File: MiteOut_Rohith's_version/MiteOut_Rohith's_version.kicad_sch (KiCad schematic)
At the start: 1 part, among them U1 ESP32-S3-WROOM-1

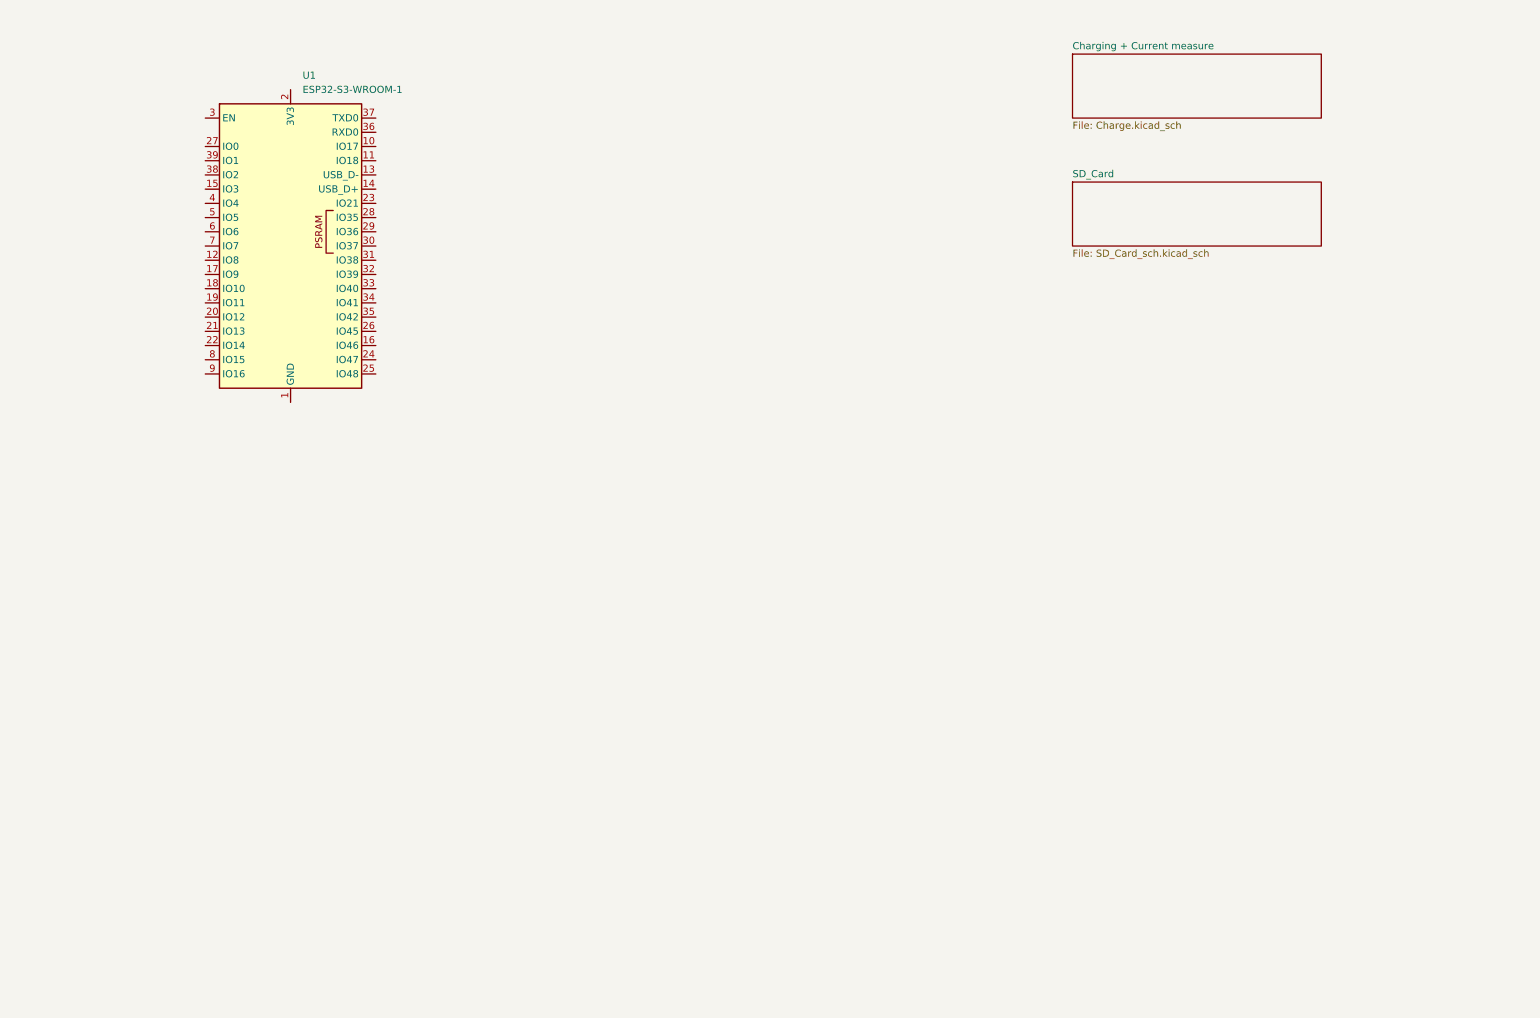
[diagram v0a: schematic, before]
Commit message: Finished ADC + ESP needing edits
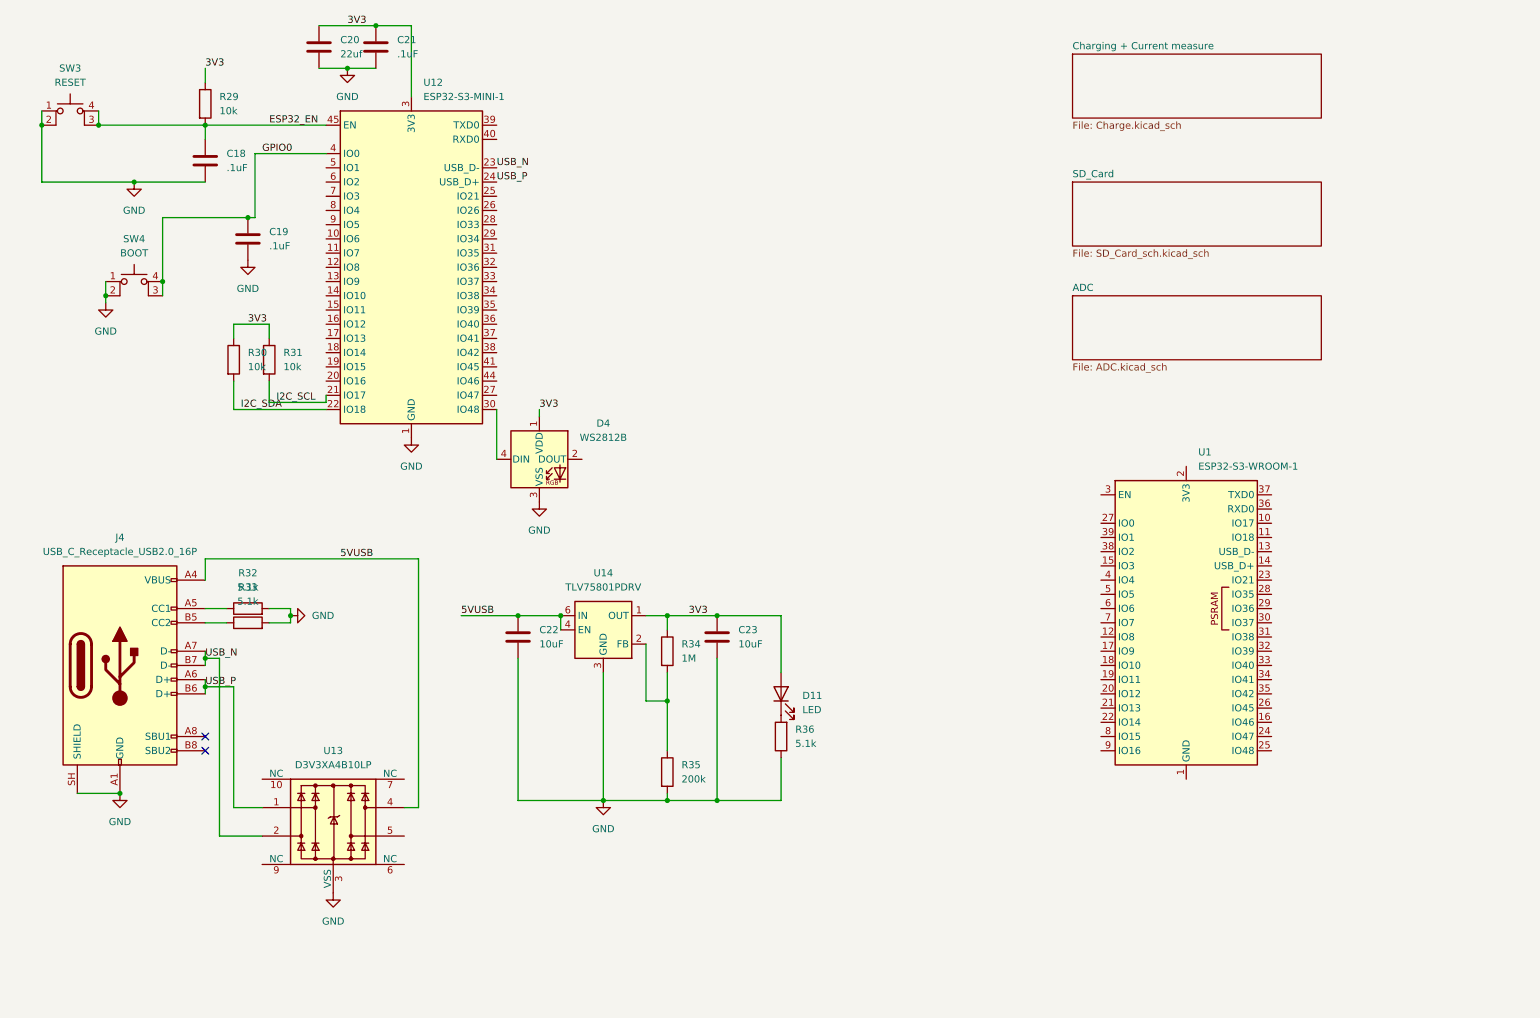
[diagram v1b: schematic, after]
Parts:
- added C18, C19, C21: .1uF, Capacitor_SMD:C_0603_1608Metric_Pad1.08x0.95mm_HandSolder, symbol Device:C
- added C20: 22uf, Capacitor_SMD:C_0603_1608Metric_Pad1.08x0.95mm_HandSolder, symbol Device:C
- added C22, C23: 10uF, symbol Device:C
- added D11: LED, LED_SMD:LED_0603_1608Metric_Pad1.05x0.95mm_HandSolder, symbol Device:LED
- added D4: WS2812B, LED_SMD:LED_WS2812B_PLCC4_5.0x5.0mm_P3.2mm, symbol LED:WS2812B
- added J4: USB_C_Receptacle_USB2.0_16P, Connector_USB:USB_C_Receptacle_GCT_USB4105-xx-A_16P_TopMnt_Horizontal, symbol Connector:USB_C_Receptacle_USB2.0_16P
- added R29, R30, R31: 10k, Resistor_SMD:R_0603_1608Metric_Pad0.98x0.95mm_HandSolder, symbol Device:R
- added R32, R33, R36: 5.1k, symbol Device:R
- added R34: 1M, Resistor_SMD:R_0603_1608Metric_Pad0.98x0.95mm_HandSolder, symbol Device:R
- added R35: 200k, Resistor_SMD:R_0603_1608Metric_Pad0.98x0.95mm_HandSolder, symbol Device:R
- added SW3: RESET, Button_Switch_SMD:SW_SPST_PTS810, symbol Switch:SW_MEC_5E
- added SW4: BOOT, Button_Switch_SMD:SW_SPST_PTS810, symbol Switch:SW_MEC_5E
- added U12: ESP32-S3-MINI-1, RF_Module:ESP32-S2-MINI-1, symbol RF_Module:ESP32-S3-MINI-1
- added U13: D3V3XA4B10LP, Package_DFN_QFN:Diodes_UDFN-10_1x2.5mm_P0.5mm, symbol Power_Protection:D3V3XA4B10LP
- added U14: TLV75801PDRV, Package_SON:WSON-6-1EP_2x2mm_P0.65mm_EP1x1.6mm, symbol Regulator_Linear:TLV75801PDRV
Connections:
- new net: R34.2, R35.1, U14.2 (FB)
- new net: J4.A5 (CC1), R32.1
- new net: J4.B5 (CC2), R33.1
- new net: D4.4 (DIN), U12.30 (IO48)
- new net: D11.1 (K), R36.2
- new net 3V3: C20.1, C21.1, C23.1, D11.2 (A), D4.1 (VDD), R29.1, R30.1, R31.1, R34.1, U12.3 (3V3), U14.1 (OUT)
- new net 5VUSB: C22.1, J4.A4 (VBUS), J4.A9 (VBUS), J4.B4 (VBUS), J4.B9 (VBUS), U13.4, U14.4 (EN), U14.6 (IN)
- new net ESP32_EN: C18.2, R29.2, SW3.3 (K), SW3.4 (A), U12.45 (EN)
- new net GND: C18.1, C19.2, C20.2, C21.2, C22.2, C23.2, D4.3 (VSS), J4.A1 (GND), J4.A12 (GND), J4.B1 (GND), J4.B12 (GND), J4.SH (SHIELD), R32.2, R33.2, R35.2, R36.1, SW3.1, SW3.2, SW4.1, SW4.2, U12.1 (GND), U12.2 (GND), U12.42 (GND), U12.43 (GND), U12.46 (GND), U12.47 (GND), U12.48 (GND), U12.49 (GND), U12.50 (GND), U12.51 (GND), U12.52 (GND), U12.53 (GND), U12.54 (GND), U12.55 (GND), U12.56 (GND), U12.57 (GND), U12.58 (GND), U12.59 (GND), U12.60 (GND), U12.61 (GND), U12.62 (GND), U12.63 (GND), U12.64 (GND), U12.65 (GND), U13.3 (VSS), U13.8 (VSS), U14.3 (GND), U14.7 (GND)
- new net GPIO0: C19.1, SW4.3 (K), SW4.4 (A), U12.4 (IO0)
- new net I2C_SCL: R31.2, U12.21 (IO17)
- new net I2C_SDA: R30.2, U12.22 (IO18)
- new net USB_N: J4.A7 (D-), J4.B7 (D-), U12.23 (USB_D-), U13.2
- new net USB_P: J4.A6 (D+), J4.B6 (D+), U12.24 (USB_D+), U13.1
- no-connect marks 0 -> 2
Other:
- added sheet ADC (ADC.kicad_sch)
- moved on the sheet: U1

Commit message: finished RTC
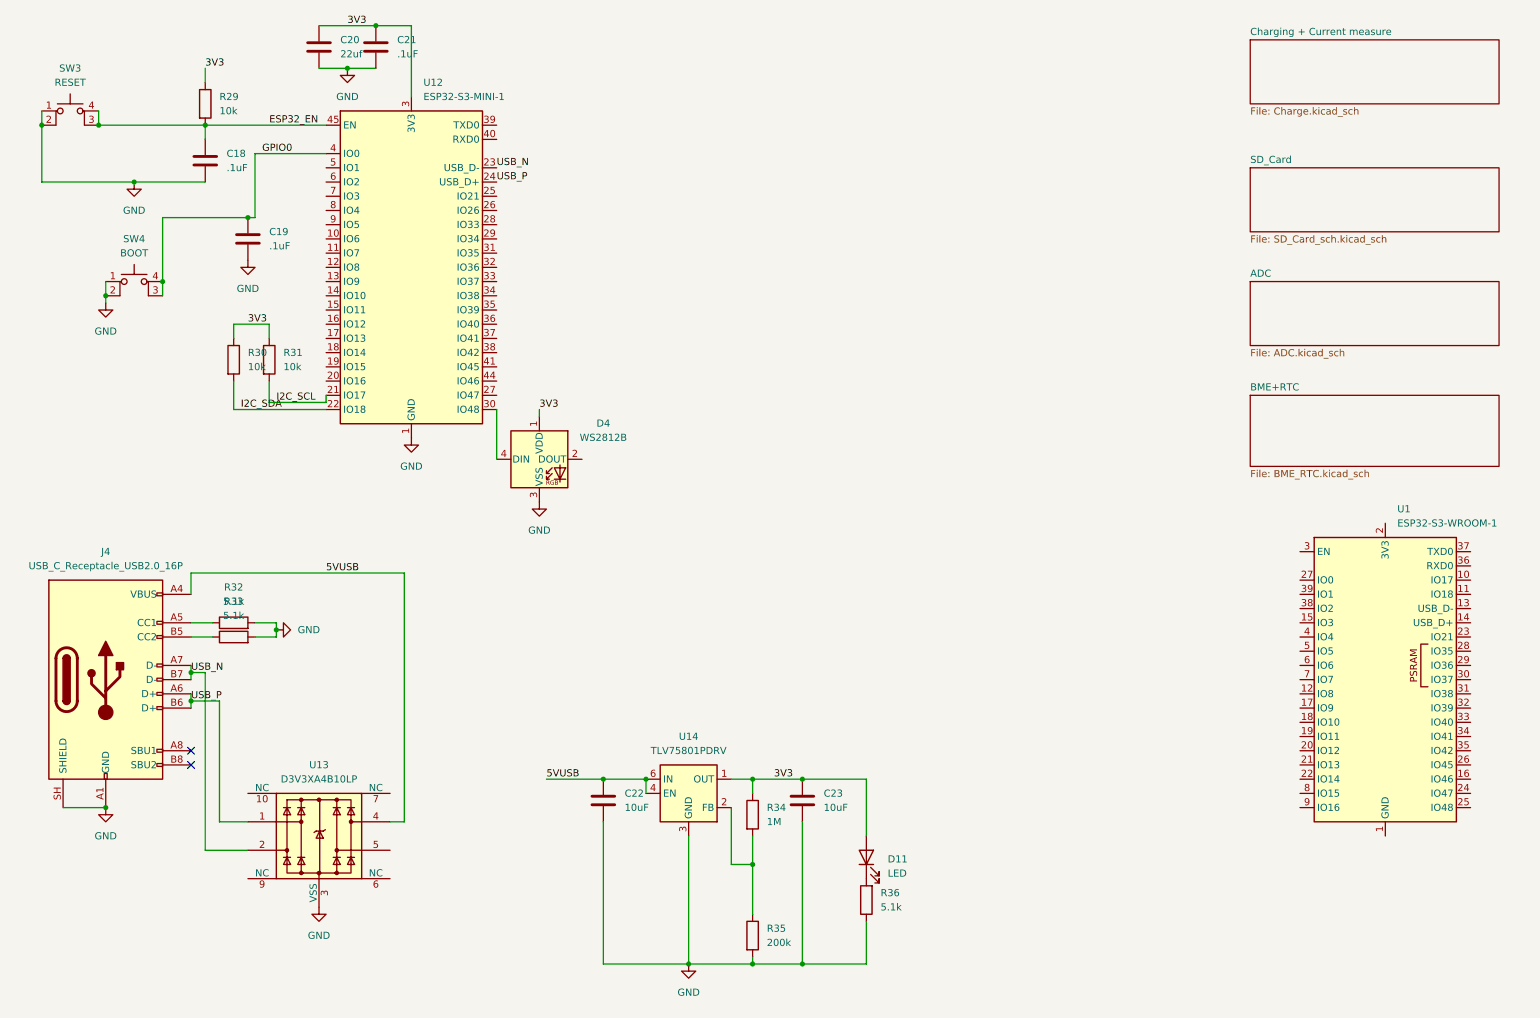
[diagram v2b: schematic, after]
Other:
- added sheet BME+RTC (BME_RTC.kicad_sch)
- moved on the sheet: C22, C23, D11, J4, R32, R33, R34, R35, R36, U1, U13, U14

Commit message: some changes ig
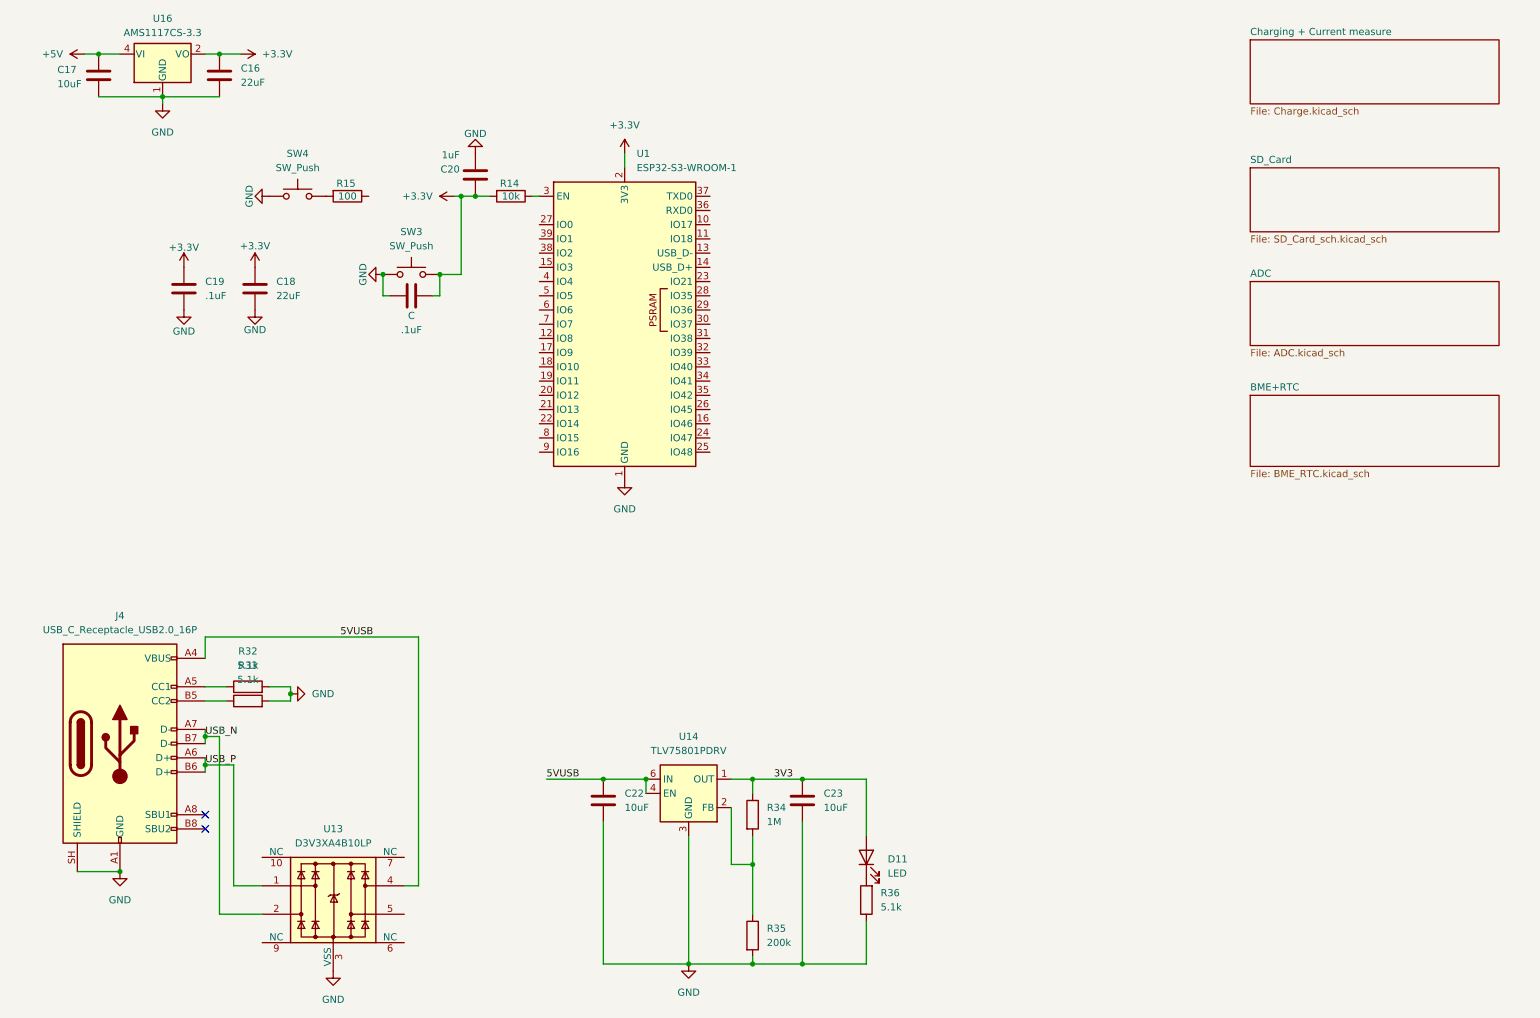
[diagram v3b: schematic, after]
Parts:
- removed C21: .1uF, Capacitor_SMD:C_0603_1608Metric_Pad1.08x0.95mm_HandSolder, symbol Device:C
- removed D4: WS2812B, LED_SMD:LED_WS2812B_PLCC4_5.0x5.0mm_P3.2mm, symbol LED:WS2812B
- removed R29, R30, R31: 10k, Resistor_SMD:R_0603_1608Metric_Pad0.98x0.95mm_HandSolder, symbol Device:R
- removed SW3: RESET, Button_Switch_SMD:SW_SPST_PTS810, symbol Switch:SW_MEC_5E
- removed SW4: BOOT, Button_Switch_SMD:SW_SPST_PTS810, symbol Switch:SW_MEC_5E
- removed U12: ESP32-S3-MINI-1, RF_Module:ESP32-S2-MINI-1, symbol RF_Module:ESP32-S3-MINI-1
- added C: .1uF, symbol Device:C
- added C16: 22uF, symbol Device:C
- added C17: 10uF, symbol Device:C
- added R14: 10k, symbol Device:R
- added R15: 100, symbol Device:R
- added SW3, SW4: SW_Push, symbol Switch:SW_Push
- added U16: AMS1117CS-3.3, Package_SO:SOIC-8_3.9x4.9mm_P1.27mm, symbol Regulator_Linear:AMS1117CS-3.3
- C18: value .1uF -> 22uF; footprint Capacitor_SMD:C_0603_1608Metric_Pad1.08x0.95mm_HandSolder -> (none)
- C19: footprint Capacitor_SMD:C_0603_1608Metric_Pad1.08x0.95mm_HandSolder -> (none)
- C20: value 22uf -> 1uF; footprint Capacitor_SMD:C_0603_1608Metric_Pad1.08x0.95mm_HandSolder -> (none)
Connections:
- net ESP32_EN is gone; now on net GND: C18.2
- net GPIO0 is gone; now on net +3.3V: C19.1
- net 3V3: no longer C20.1
- net GND: now also U1.1 (GND), U1.40 (GND), U1.41 (GND), C.1, C16.2, C17.1, SW3.1, SW4.1, U16.1 (GND); no longer C18.1
- net +3.3V: now reaches U1.2 (3V3)
- net +3.3V: now also C18.1, C20.1, C.2, C16.1, R14.2, SW3.2, U16.2 (VO), U16.3 (VO), U16.6 (VO), U16.7 (VO)
- net at U1.3 (EN): now also R14.1
- new net: R15.2, SW4.2
- new net +5V: C17.2, U16.4 (VI)
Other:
- moved on the sheet: J4, R32, R33, U1, U13

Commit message: Full Schematic Draft 1
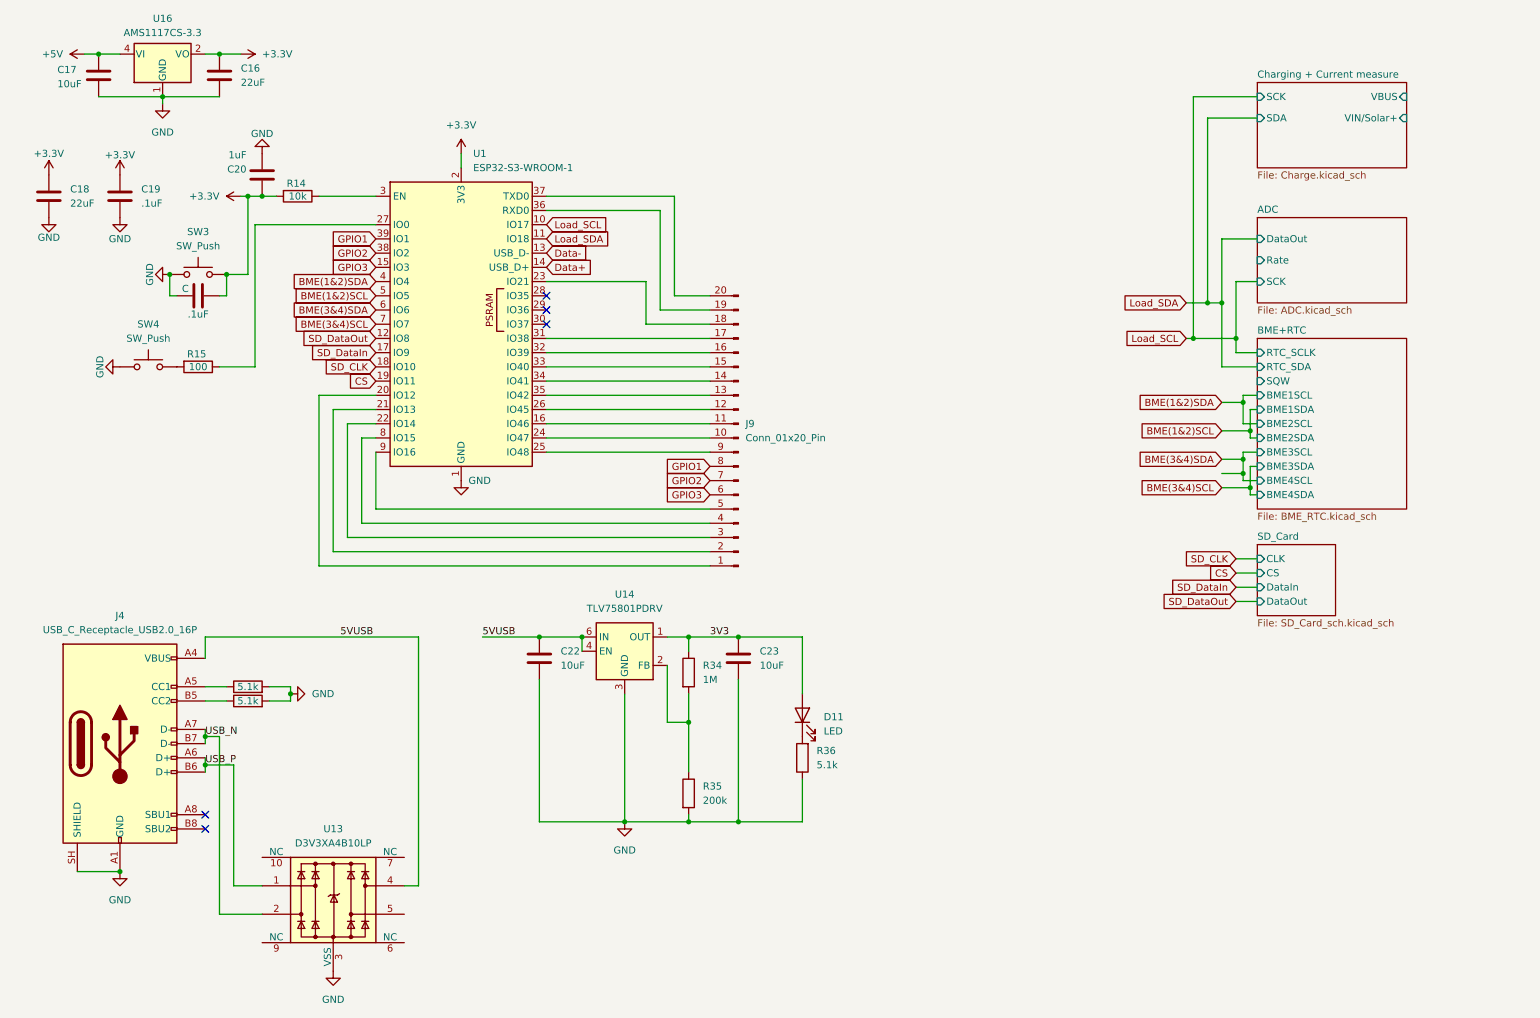
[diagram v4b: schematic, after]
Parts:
- added J9: Conn_01x20_Pin, symbol Connector:Conn_01x20_Pin
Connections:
- net Load_SCL: now reaches U1.10 (IO17)
- net Load_SDA: now reaches U1.11 (IO18)
- net SD_DataOut: now reaches U1.12 (IO8)
- net Data-: now reaches U1.13 (USB_D-)
- net Data+: now reaches U1.14 (USB_D+)
- net GPIO3: now reaches U1.15 (IO3)
- net GPIO3: now also J9.6 (Pin_6)
- net at U1.16 (IO46): now also J9.11 (Pin_11)
- net SD_DataIn: now reaches U1.17 (IO9)
- net SD_CLK: now reaches U1.18 (IO10)
- net CS: now reaches U1.19 (IO11)
- net at U1.20 (IO12): now also J9.1 (Pin_1)
- net at U1.21 (IO13): now also J9.2 (Pin_2)
- net at U1.22 (IO14): now also J9.3 (Pin_3)
- net at U1.23 (IO21): now also J9.18 (Pin_18)
- net at U1.24 (IO47): now also J9.10 (Pin_10)
- net at U1.25 (IO48): now also J9.9 (Pin_9)
- net at U1.26 (IO45): now also J9.12 (Pin_12)
- net at U1.27 (IO0): now also R15.1
- net at U1.31 (IO38): now also J9.17 (Pin_17)
- net at U1.32 (IO39): now also J9.16 (Pin_16)
- net at U1.33 (IO40): now also J9.15 (Pin_15)
- net at U1.34 (IO41): now also J9.14 (Pin_14)
- net at U1.35 (IO42): now also J9.13 (Pin_13)
- net at U1.36 (RXD0): now also J9.19 (Pin_19)
- net at U1.37 (TXD0): now also J9.20 (Pin_20)
- net GPIO2: now reaches U1.38 (IO2)
- net GPIO2: now also J9.7 (Pin_7)
- net GPIO1: now reaches U1.39 (IO1)
- net GPIO1: now also J9.8 (Pin_8)
- net BME(1&2)SDA: now reaches U1.4 (IO4)
- net BME(1&2)SCL: now reaches U1.5 (IO5)
- net BME(3&4)SDA: now reaches U1.6 (IO6)
- net BME(3&4)SCL: now reaches U1.7 (IO7)
- net at U1.8 (IO15): now also J9.4 (Pin_4)
- net at U1.9 (IO16): now also J9.5 (Pin_5)
- no-connect marks 2 -> 5
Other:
- sheet ADC ports: added DataOut, Rate, SCK; removed none
- sheet BME+RTC ports: added BME1SCL, BME1SDA, BME2SCL, BME2SDA, BME3SCL, BME3SDA, BME4SCL, BME4SDA, RTC_SCLK, RTC_SDA, SQW; removed none
- sheet Charging + Current measure ports: added SCK, SDA, VBUS, VIN/Solar+; removed none
- sheet SD_Card ports: added CLK, CS, DataIn, DataOut; removed none
- moved on the sheet: C, C18, C19, C20, C22, C23, D11, R14, R15, R34, R35, R36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
